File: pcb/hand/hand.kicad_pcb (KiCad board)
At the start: 2 copper layers, 149.5 x 99.8 mm, 35 parts, among them J1 Conn_01x15, J2 Conn_01x15

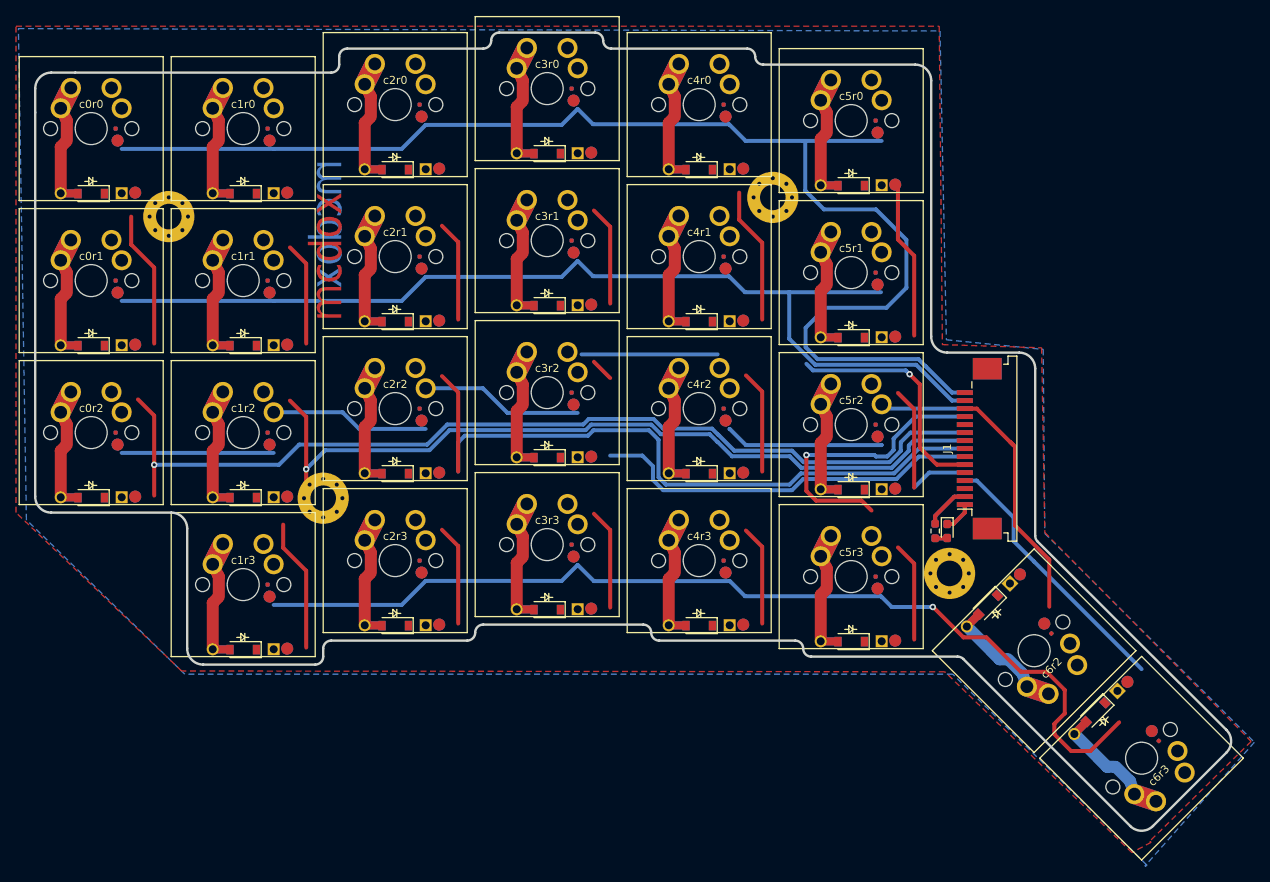
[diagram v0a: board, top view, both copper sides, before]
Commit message: pcb/hand Full layout.
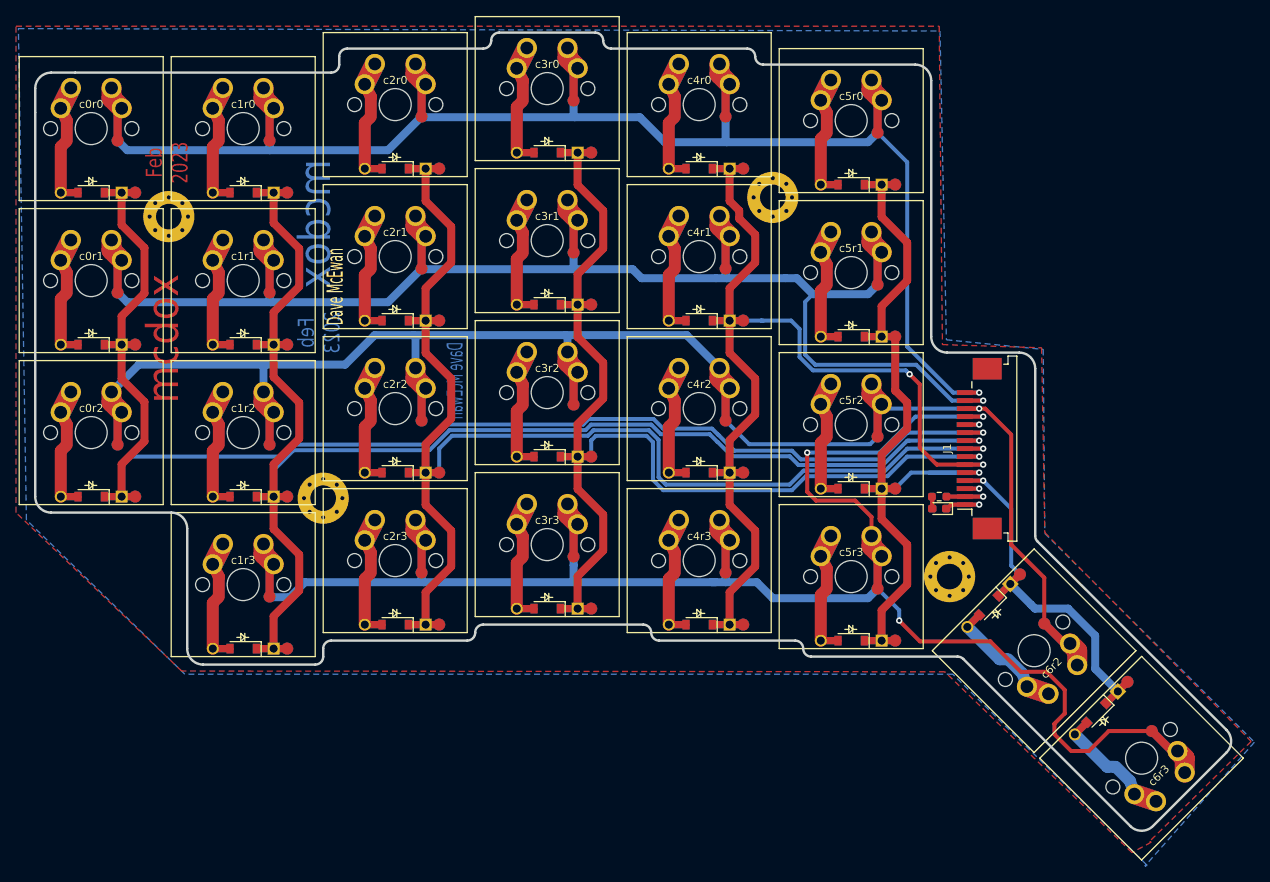
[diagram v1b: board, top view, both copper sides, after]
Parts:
- moved R1 4.33 mm to (113.0, 53.0), turned to 180 degrees
- moved R2 4.33 mm to (113.0, 53.0), turned to 180 degrees
- moved LED1 2.97 mm to (113.0, 54.5), turned to 180 degrees
- moved LED2 2.97 mm to (113.0, 54.5), turned to 180 degrees
- moved H4 0.40 mm to (114.3, 63.0)
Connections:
- J1 pad 11: (no net) -> row4_NC
- J1 pad 3: (no net) -> col7_NC
- J2 pad 13: (no net) -> col7_NC
- J2 pad 5: (no net) -> row4_NC
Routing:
- net row2: track 136.5 -> 237.7 mm, vias 0 -> 1
- net row3: track 160.4 -> 246.1 mm, vias 2 -> 3
- net col3: track 76.8 -> 155.6 mm, vias 0 -> 1
- net row1: track 129.6 -> 208.1 mm, vias 0 -> 1
- net col4: track 72.1 -> 142.4 mm, vias 1 -> 2
- net col2: track 113.0 -> 177.4 mm, vias 0 -> 1
- net col1: track 130.8 -> 194.8 mm
- net col5: track 51.8 -> 112.7 mm, vias 0 -> 1
- net row0: track 165.5 -> 216.8 mm, vias 0 -> 1
- net col0: track 138.0 -> 185.6 mm
- net col6: track 33.6 -> 55.0 mm, vias 0 -> 1
- net row4_NC: track 0.00 -> 3.60 mm, vias 0 -> 1
- net col7_NC: track 0.00 -> 3.60 mm, vias 0 -> 1
- net +3V3: track 11.4 -> 9.18 mm, vias 0 -> 1
- net GND: track 7.58 -> 8.66 mm, vias 0 -> 1
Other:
- board text added: "Dave McEwan"
- board text added: "Feb 2023"
